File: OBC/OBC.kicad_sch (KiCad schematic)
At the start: 9 parts, among them J2 IDC1 (PMS-Raspi), J3 IDC2 (Raspi-TRU), J4 IDC3 (Modo operación), J5 Conn_01x04, U1 MPU9250, U2 BMP280, U3 RASPBERRY_PI_ZERO_2_W

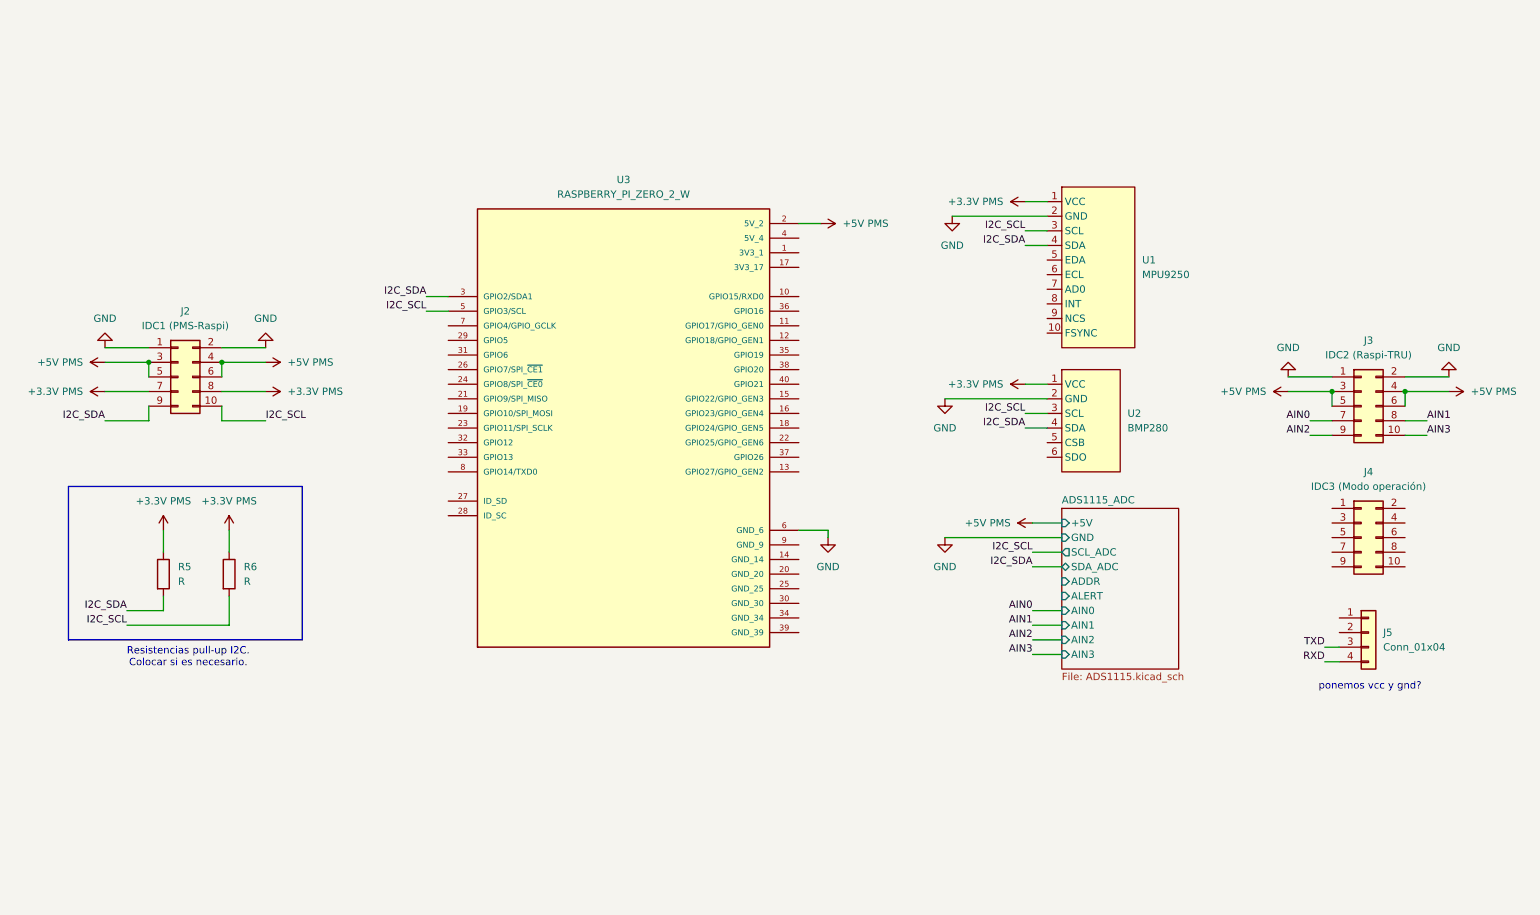
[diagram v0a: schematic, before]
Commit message: Organiza sch general
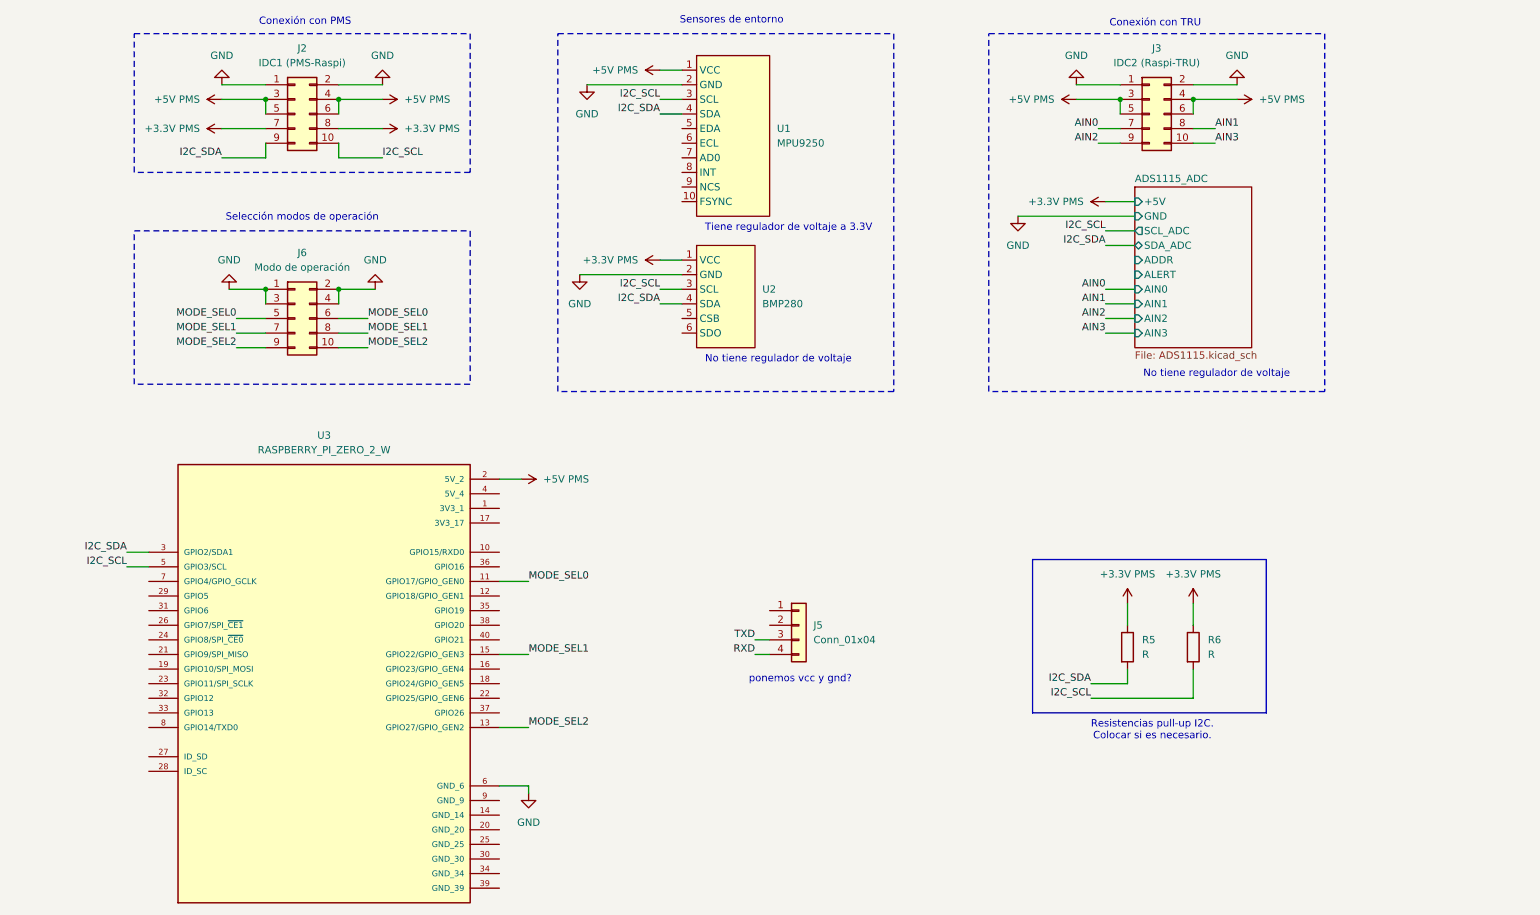
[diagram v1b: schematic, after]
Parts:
- removed J4: IDC3 (Modo operación), symbol Connector_Generic:Conn_02x05_Odd_Even
- added J6: Modo de operación, symbol Connector_Generic:Conn_02x05_Odd_Even
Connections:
- net +3.3V PMS: no longer U1.1 (VCC)
- net +5V PMS: now also U1.1 (VCC)
- net GND: now also J6.1 (Pin_1), J6.2 (Pin_2), J6.3 (Pin_3), J6.4 (Pin_4)
- net MODE_SEL0: now reaches U3.11 (GPIO17/GPIO_GEN0)
- net MODE_SEL0: now also J6.5 (Pin_5), J6.6 (Pin_6)
- net MODE_SEL2: now reaches U3.13 (GPIO27/GPIO_GEN2)
- net MODE_SEL2: now also J6.10 (Pin_10), J6.9 (Pin_9)
- net MODE_SEL1: now reaches U3.15 (GPIO22/GPIO_GEN3)
- net MODE_SEL1: now also J6.7 (Pin_7), J6.8 (Pin_8)
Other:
- note added: "Conexión con PMS"
- note added: "Conexión con TRU"
- note added: "No tiene regulador de voltaje"
- note added: "Selección modos de operación"
- note added: "Sensores de entorno"
- note added: "Tiene regulador de voltaje a 3.3V"
- moved on the sheet: J2, J3, J5, R5, R6, U1, U2, U3
